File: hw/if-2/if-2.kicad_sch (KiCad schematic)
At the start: 4 parts

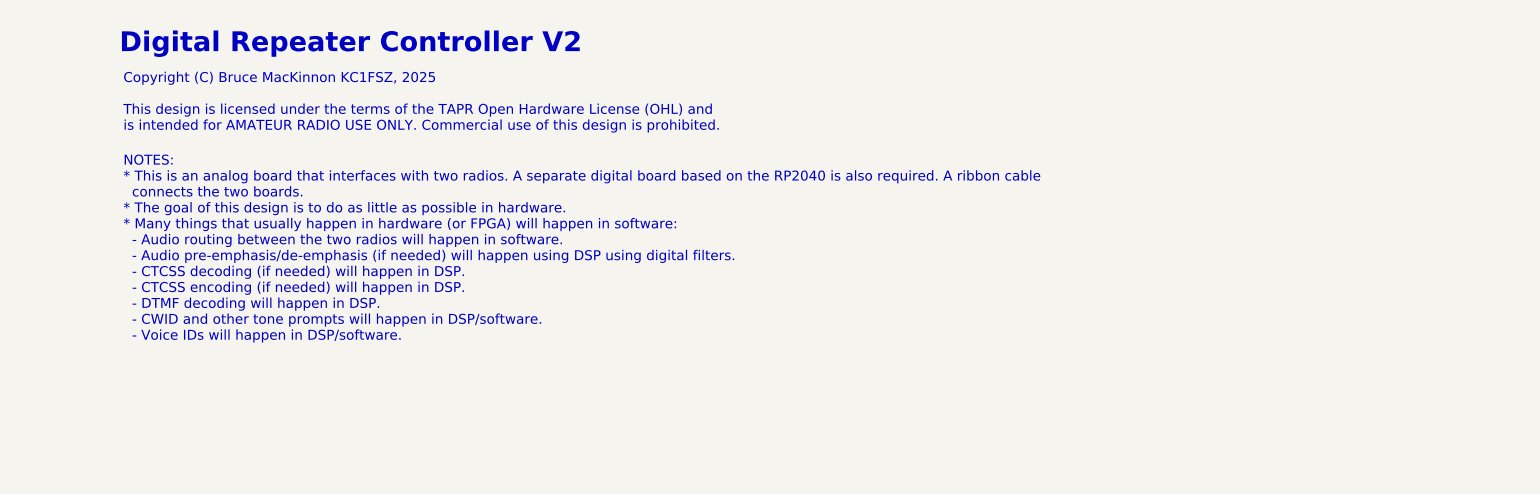
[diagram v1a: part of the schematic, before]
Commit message: Docs
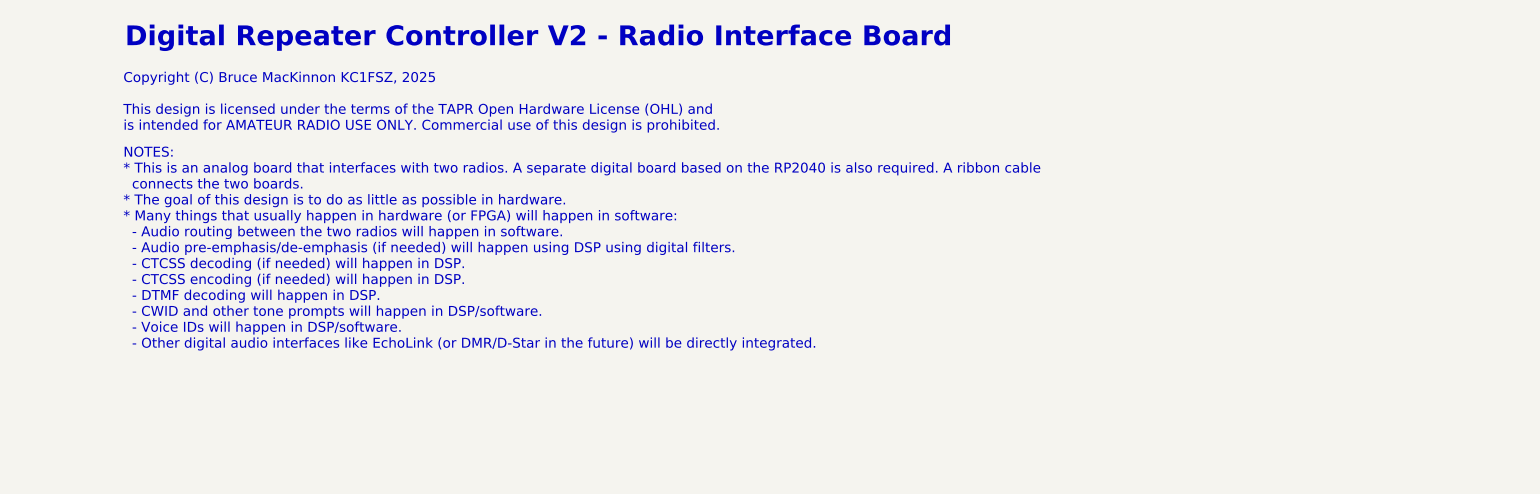
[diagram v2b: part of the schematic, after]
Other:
- note added: "Digital Repeater Controller V2 - Radio Interface Board"
- note removed: "Digital Repeater Controller V2"
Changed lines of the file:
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@@
 		)
 	)
-	(text "Digital Repeater Controller V2"
+	(text "Digital Repeater Controller V2 - Radio Interface Board"
 		(exclude_from_sim no)
-		(at 47.244 21.844 0)
+		(at 71.374 21.082 0)
 		(effects
 			(font
@@
 		)
 	)
-	(text "NOTES:\n* This is an analog board that interfaces with two radios. A separate digital board based on the RP2040 is also required. A ribbon cable\n  connects the two boards.\n* The goal of this design is to do as little as possible in hardware.\n* Many things that usually happen in hardware (or FPGA) will happen in software:\n  - Audio routing between the two radios will happen in software.\n  - Audio pre-emphasis/de-emphasis (if needed) will happen using DSP using digital filters.\n  - CTCSS decoding (if needed) will happen in DSP.\n  - CTCSS encoding (if needed) will happen in DSP.\n  - DTMF decoding will happen in DSP.\n  - CWID and other tone prompts will happen in DSP/software.\n  - Voice IDs will happen in DSP/software.\n\n"
+	(text "NOTES:\n* This is an analog board that interfaces with two radios. A separate digital board based on the RP2040 is also required. A ribbon cable\n  connects the two boards.\n* The goal of this design is to do as little as possible in hardware.\n* Many things that usually happen in hardware (or FPGA) will happen in software:\n  - Audio routing between the two radios will happen in software.\n  - Audio pre-emphasis/de-emphasis (if needed) will happen using DSP using digital filters.\n  - CTCSS decoding (if needed) will happen in DSP.\n  - CTCSS encoding (if needed) will happen in DSP.\n  - DTMF decoding will happen in DSP.\n  - CWID and other tone prompts will happen in DSP/software.\n  - Voice IDs will happen in DSP/software.\n  - Other digital audio interfaces like EchoLink (or DMR/D-Star in the future) will be directly integrated.\n\n"
 		(exclude_from_sim no)
 		(at 18.034 49.276 0)

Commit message: Ready to do layout on IF2 board
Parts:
- H1, H2, H3, H4: footprint (none) -> MountingHole:MountingHole_3.5mm
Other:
- title: Digital Repeater Controller  -> COS/CTCSS/PTT Controls (Radio 1)
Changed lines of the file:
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@@
 	(paper "USLetter")
 	(title_block
-		(title "Digital Repeater Controller ")
+		(title "COS/CTCSS/PTT Controls (Radio 1)")
 		(date "2025-03-18")
 		(rev "2")
@@
 			)
 		)
-		(property "Footprint" ""
+		(property "Footprint" "MountingHole:MountingHole_3.5mm"
 			(at 133.35 186.69 0)
 			(effects
@@
 			)
 		)
-		(property "Footprint" ""
+		(property "Footprint" "MountingHole:MountingHole_3.5mm"
 			(at 133.35 180.34 0)
 			(effects
@@
 			)
 		)
-		(property "Footprint" ""
+		(property "Footprint" "MountingHole:MountingHole_3.5mm"
 			(at 133.35 193.04 0)
 			(effects
@@
 			)
 		)
-		(property "Footprint" ""
+		(property "Footprint" "MountingHole:MountingHole_3.5mm"
 			(at 133.35 173.99 0)
 			(effects

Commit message: Making progress on layout
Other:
- title: COS/CTCSS/PTT Controls (Radio 1) -> Title Page
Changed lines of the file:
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@@
 	(paper "USLetter")
 	(title_block
-		(title "COS/CTCSS/PTT Controls (Radio 1)")
-		(date "2025-03-18")
+		(title "Title Page")
+		(date "2025-05-09")
 		(rev "2")
 		(company "Bruce MacKinnon KC1FSZ")
